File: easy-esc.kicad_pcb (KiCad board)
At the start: 2 copper layers, 43 parts, among them J101 USB_C_Receptacle_USB2.0, J102 BLDC, J103 POWER, SW101 BOOT, SW102 RESET, SW103 EN, U101 TMC6300, U102 XC6206, U103 W25Q128JVS, U104 RP2040, Y101 12MHz

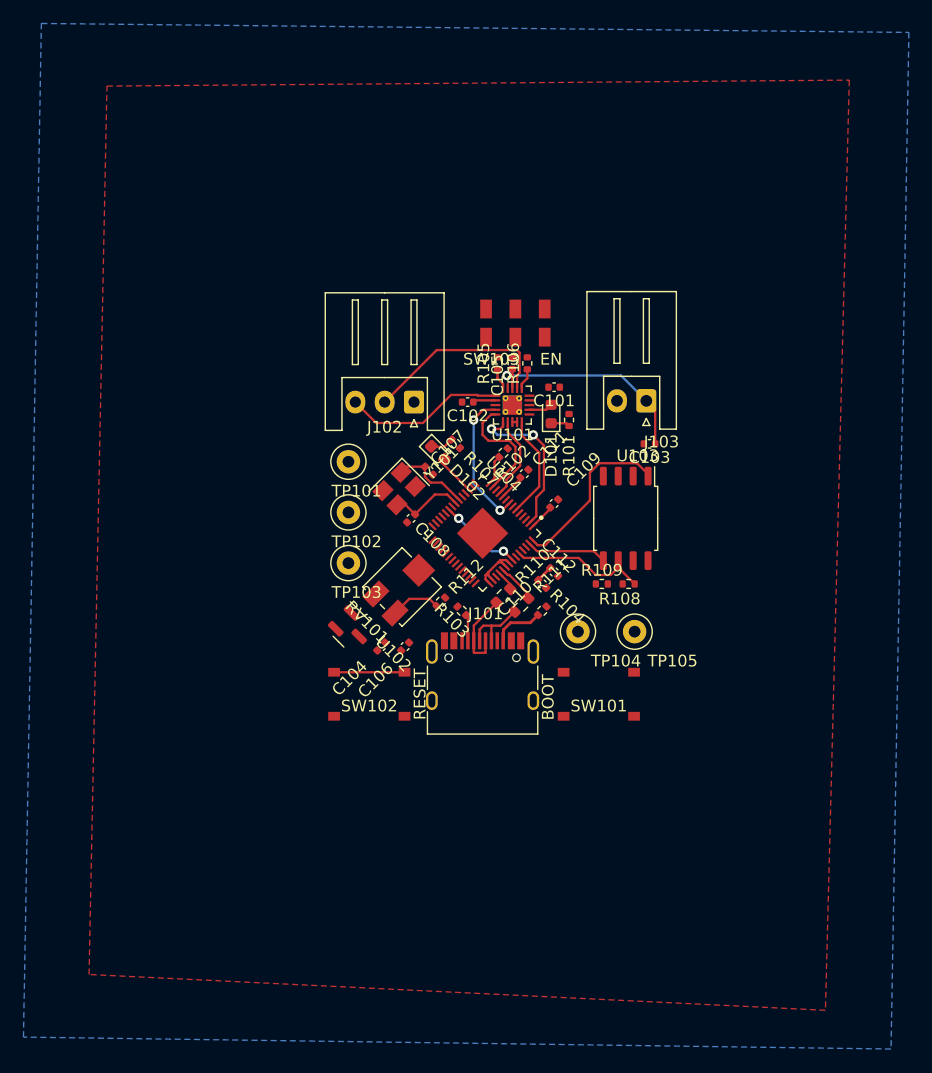
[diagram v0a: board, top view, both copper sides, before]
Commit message: finalize fab files
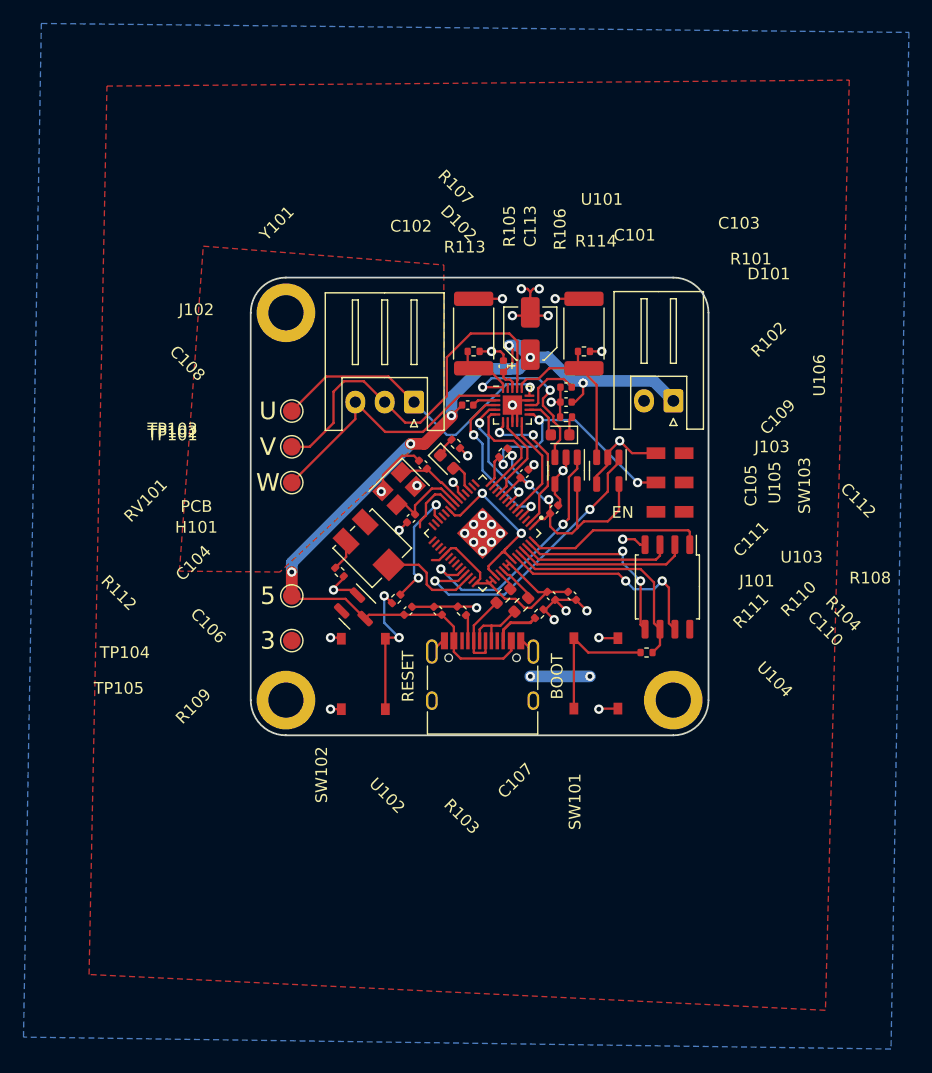
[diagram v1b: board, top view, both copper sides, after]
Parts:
- added C113: 100uF, Capacitor_SMD:CP_Elec_4x3.9, F.Cu at (137.4, 105.7)
- added G***: LOGO, matei:happymeal, B.Cu at (133.3, 118.4)
- added H101: PCB, matei:easy-esc-outline, F.Cu at (133.1, 120.4)
- added R113: 0, Resistor_SMD:R_0402_1005Metric, F.Cu at (132.6, 107.2)
- added R114: 0, Resistor_SMD:R_0402_1005Metric, F.Cu at (142.0, 107.2)
- added U105: INA180A1, Package_TO_SOT_SMD:SOT-23-5, F.Cu at (140.5, 117.3)
- added U106: INA180A1, Package_TO_SOT_SMD:SOT-23-5, F.Cu at (144.0, 117.3)
- R105, R106: footprint Resistor_SMD:R_0402_1005Metric -> Resistor_SMD:R_2512_6332Metric
- TP101, TP102, TP103, TP104, TP105: footprint TestPoint:TestPoint_Loop_D1.80mm_Drill1.0mm_Beaded -> TestPoint:TestPoint_Pad_D1.5mm
- U101: footprint Package_DFN_QFN:QFN-20-1EP_3x3mm_P0.4mm_EP1.65x1.65mm_ThermalVias -> Package_DFN_QFN:QFN-20-1EP_3x3mm_P0.4mm_EP1.65x1.65mm
- moved TP105 29.2 mm to (117.1, 131.8)
- moved TP104 24.6 mm to (117.1, 128.0)
- moved SW103 18.5 mm to (147.3, 117.9), turned to -90 degrees
- moved R109 17.6 mm to (126.0, 128.3), turned to -135 degrees
- moved R112 9.00 mm to (121.2, 126.0), turned to 135 degrees
- moved TP103 8.39 mm to (117.1, 118.4)
- moved C103 7.95 mm to (140.5, 111.5)
- moved TP102 7.38 mm to (117.1, 115.3)
- moved U103 6.84 mm to (149.1, 127.3)
- moved TP101 6.48 mm to (117.1, 112.3)
- moved R108 6.04 mm to (147.3, 132.8)
- moved R106 5.45 mm to (142.0, 105.7)
- moved RV101 4.17 mm to (124.0, 124.0), turned to 45 degrees
- moved C106 4.13 mm to (129.5, 129.3), turned to 135 degrees
- moved C104 3.81 mm to (127.0, 129.3), turned to 45 degrees
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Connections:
- U101 pad 21: (no net) -> GND
- U104 pad 38: WSENSE -> WCUR
- U104 pad 39: UVSENSE -> UVCUR
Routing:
- net GND: track 0.40 -> 71.3 mm, vias 0 -> 37
- net +5V: track 18.8 -> 78.9 mm, vias 1 -> 6
- net +3V3: track 11.1 -> 57.6 mm, vias 0 -> 5
- net Net-(J102-Pad1): track 0.51 -> 26.2 mm, vias 0 -> 1
- net UVCUR: track 0.00 -> 25.1 mm, vias 0 -> 2
- net WCUR: track 0.00 -> 21.9 mm, vias 0 -> 2
- net CLEAR: track 2.57 -> 23.3 mm, vias 0 -> 3
- net QD3: track 0.00 -> 18.4 mm, vias 0 -> 2
- net WSENSE: track 1.79 -> 20.2 mm, vias 0 -> 2
- net Net-(J102-Pad2): track 16.7 -> 33.9 mm
- net QD0: track 0.00 -> 14.7 mm
- net UVSENSE: track 1.79 -> 15.9 mm
- net UH: track 0.00 -> 13.9 mm, vias 0 -> 2
- net QD2: track 0.00 -> 12.9 mm
- net Net-(R108-Pad2): track 0.00 -> 12.2 mm
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- added copper zone on F.Cu, net GND
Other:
- board outline added: 39 x 39 mm
- board text added: "3"
- board text added: "5"
- board text added: "U"
- board text added: "V"
- board text added: "W"
- board text added: "mateijordache"
